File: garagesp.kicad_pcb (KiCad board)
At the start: 2 copper layers, 45 x 45 mm, 21 parts, among them J1 USB_C_Receptacle_USB2.0_14P, J2 AHT21, J3 DOOR CTL, J4 DOOR SW, K1 SANYOU_SRD_Form_A, Q1 BC547, SW1 RESET, SW2 BOOT, U1 ESP32-C3-WROOM-02, U2 AP2112K-3.3

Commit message: add capacitors and resistors
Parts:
- removed C1, C2: 10uF, Capacitor_SMD:C_0805_2012Metric_Pad1.18x1.45mm_HandSolder
- removed C3: 100 nF, Capacitor_SMD:C_0805_2012Metric_Pad1.18x1.45mm_HandSolder
- removed D1: B120-E3, Diode_SMD:D_SMA
- removed J1: USB_C_Receptacle_USB2.0_14P, Connector_USB:USB_C_Receptacle_HCTL_HC-TYPE-C-16P-01A
- removed J2: AHT21, Connector_PinHeader_2.54mm:PinHeader_1x04_P2.54mm_Vertical
- removed J3: DOOR CTL, Connector_Molex:Molex_Micro-Fit_3.0_43650-0200_1x02_P3.00mm_Horizontal
- removed J4: DOOR SW, Connector_Molex:Molex_Micro-Fit_3.0_43650-0200_1x02_P3.00mm_Horizontal
- removed K1: SANYOU_SRD_Form_A, Relay_THT:Relay_SPST_SANYOU_SRD_Series_Form_A
- removed Q1: BC547, Package_TO_SOT_THT:TO-92_Inline
- removed R1, R2, R7: 5.1k, Resistor_SMD:R_0805_2012Metric_Pad1.20x1.40mm_HandSolder
- removed R3, R4, R5, R6: 10k, Resistor_SMD:R_0805_2012Metric_Pad1.20x1.40mm_HandSolder
- removed SW1: RESET, Button_Switch_SMD:SW_SPST_TS-1088-xR020
- removed SW2: BOOT, Button_Switch_SMD:SW_SPST_TS-1088-xR020
- removed U1: ESP32-C3-WROOM-02, RF_Module:ESP32-C3-WROOM-02
- removed U2: AP2112K-3.3, Package_TO_SOT_SMD:SOT-23-5
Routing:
- net /3V3: track 59.7 -> 0.00 mm
- net GND: track 51.2 -> 0.00 mm, vias 1 -> 0
- net /SW: track 33.7 -> 0.00 mm
- net /5V: track 29.6 -> 0.00 mm, vias 3 -> 0
- net Net-(Q1-B): track 25.5 -> 0.00 mm
- net /CTL1: track 23.0 -> 0.00 mm
- net Net-(U1-EN): track 21.2 -> 0.00 mm
- net /CTL2: track 15.8 -> 0.00 mm
- net Net-(U1-IO2): track 13.5 -> 0.00 mm
- net Net-(U1-IO8): track 10.2 -> 0.00 mm
- net /SCL: track 9.87 -> 0.00 mm
- net /RELAY: track 9.21 -> 0.00 mm
- net Net-(D1-K): track 8.99 -> 0.00 mm
- net Net-(U1-IO9): track 8.86 -> 0.00 mm
- net /D+: track 7.56 -> 0.00 mm
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- removed copper zone on B.Cu, net GND
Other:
- board outline removed

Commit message: new pcb design
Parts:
- added C1: 10uF, Capacitor_SMD:C_0603_1608Metric_Pad1.08x0.95mm_HandSolder, F.Cu at (105.2, 71.5)
- added C10: 100nF, Capacitor_SMD:C_0603_1608Metric_Pad1.08x0.95mm_HandSolder, F.Cu at (98.6, 67.4)
- added C11: 4.7uF, Capacitor_SMD:CP_Elec_4x5.4, F.Cu at (103.0, 67.5)
- added C2: 10uF, Capacitor_SMD:C_0603_1608Metric_Pad1.08x0.95mm_HandSolder, F.Cu at (92.5, 69.0)
- added C3: 100nF, Capacitor_SMD:C_0603_1608Metric_Pad1.08x0.95mm_HandSolder, F.Cu at (90.8, 69.0)
- added C4: 10uF, Capacitor_SMD:C_0603_1608Metric_Pad1.08x0.95mm_HandSolder, F.Cu at (68.5, 51.8)
- added C5: 100nF, Capacitor_SMD:C_0603_1608Metric_Pad1.08x0.95mm_HandSolder, F.Cu at (66.5, 51.8)
- added C6: 10uF, Capacitor_SMD:C_0603_1608Metric_Pad1.08x0.95mm_HandSolder, F.Cu at (76.5, 69.5)
- added C7: 100nF, Capacitor_SMD:C_0603_1608Metric_Pad1.08x0.95mm_HandSolder, F.Cu at (78.2, 69.5)
- added C9: 10nF, Capacitor_SMD:C_0603_1608Metric_Pad1.08x0.95mm_HandSolder, F.Cu at (100.6, 61.2)
- added D1: B120-E3, Diode_SMD:D_SMA, F.Cu at (90.5, 72.5)
- added D2: RED LED, LED_SMD:LED_0603_1608Metric_Pad1.05x0.95mm_HandSolder, F.Cu at (108.8, 80.5)
- added D3: GREEN LED, LED_SMD:LED_0603_1608Metric_Pad1.05x0.95mm_HandSolder, F.Cu at (107.0, 80.5)
- added D4: GREEN LED, LED_SMD:LED_0603_1608Metric_Pad1.05x0.95mm_HandSolder, F.Cu at (69.4, 80.0)
- added D5: GREEN LED, LED_SMD:LED_0603_1608Metric_Pad1.05x0.95mm_HandSolder, F.Cu at (55.9, 76.2)
- added FB1: 70mΩ 33Ω@100MHz, Inductor_SMD:L_0805_2012Metric_Pad1.05x1.20mm_HandSolder, F.Cu at (98.6, 63.5)
- added J1: USB_C_Receptacle_USB2.0_14P, Connector_USB:USB_C_Receptacle_HCTL_HC-TYPE-C-16P-01A, F.Cu at (106.5, 58.0)
- added J2: AHT21, Connector_PinSocket_2.54mm:PinSocket_1x04_P2.54mm_Vertical, F.Cu at (62.5, 52.2)
- added J3: DOOR CTL, Connector_Molex:Molex_Micro-Fit_3.0_43650-0200_1x02_P3.00mm_Horizontal, F.Cu at (101.8, 85.4)
- added J4: DOOR SW, Connector_Molex:Molex_Micro-Fit_3.0_43650-0200_1x02_P3.00mm_Horizontal, F.Cu at (58.0, 85.4)
- added K1: SANYOU_SRD_Form_A, Relay_THT:Relay_SPST_SANYOU_SRD_Series_Form_A, F.Cu at (86.5, 76.0)
- added Q1: SS8050, Package_TO_SOT_SMD:SOT-23, F.Cu at (76.1, 81.5)
- added Q2: SS8050, Package_TO_SOT_SMD:SOT-23, F.Cu at (56.8, 79.2)
- added R1: 5.1k, Resistor_SMD:R_0603_1608Metric_Pad0.98x0.95mm_HandSolder, F.Cu at (103.4, 51.8)
- added R10: 1k, Resistor_SMD:R_0603_1608Metric_Pad0.98x0.95mm_HandSolder, F.Cu at (76.1, 78.7)
- added R11: 220, Resistor_SMD:R_0603_1608Metric_Pad0.98x0.95mm_HandSolder, F.Cu at (52.5, 79.0)
- added R12: 220, Resistor_SMD:R_0603_1608Metric_Pad0.98x0.95mm_HandSolder, F.Cu at (107.0, 77.0)
- added R13: 10k, Resistor_SMD:R_0603_1608Metric_Pad0.98x0.95mm_HandSolder, F.Cu at (52.5, 80.5)
- added R14: 220, Resistor_SMD:R_0603_1608Metric_Pad0.98x0.95mm_HandSolder, F.Cu at (108.8, 77.0)
- added R2: 5.1k, Resistor_SMD:R_0603_1608Metric_Pad0.98x0.95mm_HandSolder, F.Cu at (103.4, 64.2)
- added R3: 10k, Resistor_SMD:R_0603_1608Metric_Pad0.98x0.95mm_HandSolder, F.Cu at (76.5, 66.0)
- added R4: 10k, Resistor_SMD:R_0603_1608Metric_Pad0.98x0.95mm_HandSolder, F.Cu at (83.8, 66.0)
- added R5: 10k, Resistor_SMD:R_0603_1608Metric_Pad0.98x0.95mm_HandSolder, F.Cu at (78.2, 66.0)
- added R6: 10k, Resistor_SMD:R_0603_1608Metric_Pad0.98x0.95mm_HandSolder, F.Cu at (73.8, 65.1)
- added R7: 100, Resistor_SMD:R_0603_1608Metric_Pad0.98x0.95mm_HandSolder, F.Cu at (67.5, 61.8)
- added R8: 2.2k, Resistor_SMD:R_0603_1608Metric_Pad0.98x0.95mm_HandSolder, F.Cu at (58.8, 59.9)
- added R9: 2.2k, Resistor_SMD:R_0603_1608Metric_Pad0.98x0.95mm_HandSolder, F.Cu at (58.8, 57.3)
- added SW1: ~, Button_Switch_SMD:SW_SPST_TS-1088-xR020, F.Cu at (81.0, 69.0)
- added SW2: ~, Button_Switch_SMD:SW_SPST_TS-1088-xR020, F.Cu at (73.8, 69.0)
- added U1: ESP32-C3-WROOM-02, RF_Module:ESP32-C3-WROOM-02, F.Cu at (79.4, 56.8)
- added U2: AMS1117-3.3, Package_TO_SOT_SMD:SOT-223-3_TabPin2, F.Cu at (99.0, 73.8)
- added U3: USBLC6-2SC6, Package_TO_SOT_SMD:SOT-23-6, F.Cu at (97.6, 58.0)
- added U4: PC817, Package_DIP:DIP-4_W7.62mm, F.Cu at (69.4, 73.7)
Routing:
- net +3V3: track 0.00 -> 114.7 mm
- net /SW: track 0.00 -> 28.7 mm
- net /EN: track 0.00 -> 24.8 mm
- net /CTL2: track 0.00 -> 20.3 mm
- net /CTL1: track 0.00 -> 19.2 mm
- net +5V: track 0.00 -> 17.9 mm
- net Net-(U3-VBUS): track 0.00 -> 16.8 mm
- net Net-(D1-A): track 0.00 -> 15.1 mm
- net Net-(U1-IO2): track 0.00 -> 13.5 mm
- net /SDA: track 0.00 -> 12.9 mm
- net GND: track 0.00 -> 12.9 mm, vias 0 -> 41
- net /BOOT: track 0.00 -> 12.5 mm
- net /SCL: track 0.00 -> 12.4 mm
- net Net-(R7-Pad1): track 0.00 -> 11.9 mm
- net Net-(U1-IO18): track 0.00 -> 8.63 mm
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- added copper zone on B.Cu, net GND
- added copper zone on F.Cu, net GND
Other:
- board outline added: 60 x 45 mm

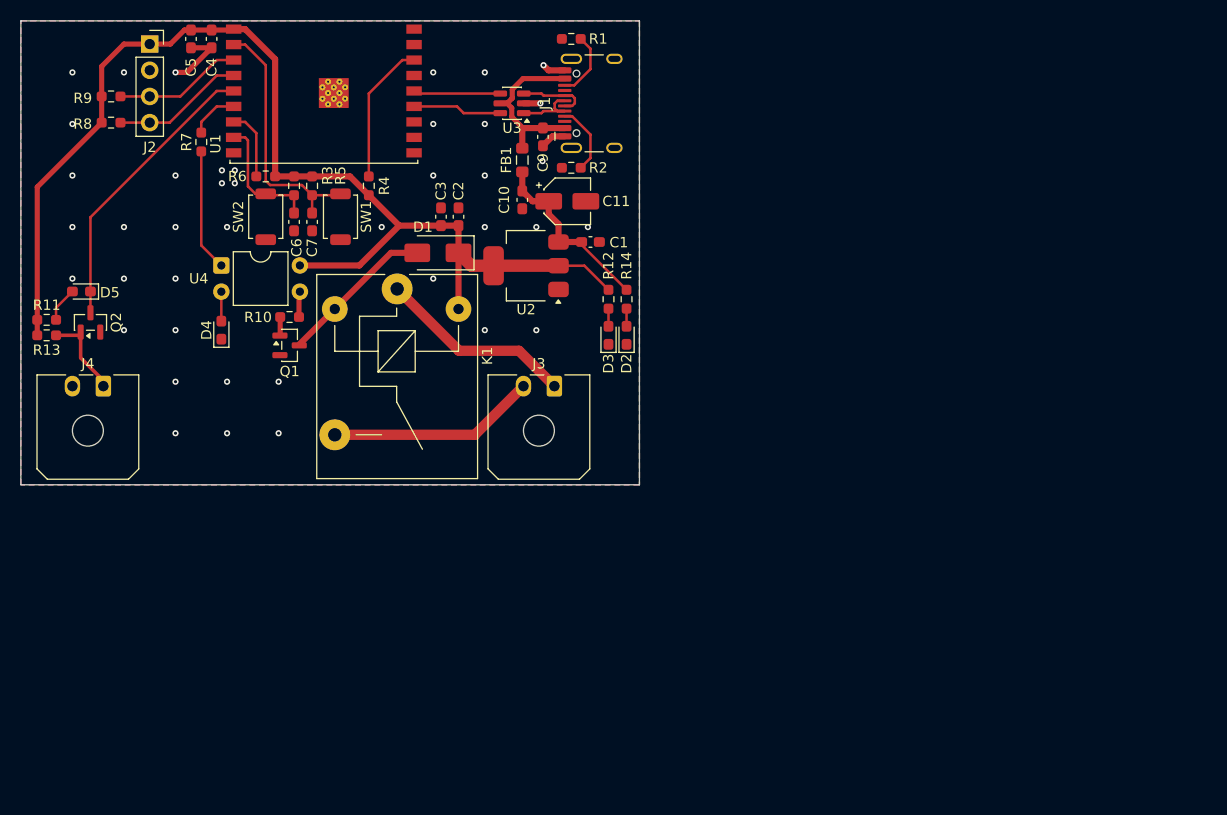
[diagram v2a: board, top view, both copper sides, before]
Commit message: I like this but want to invert my input LEDs
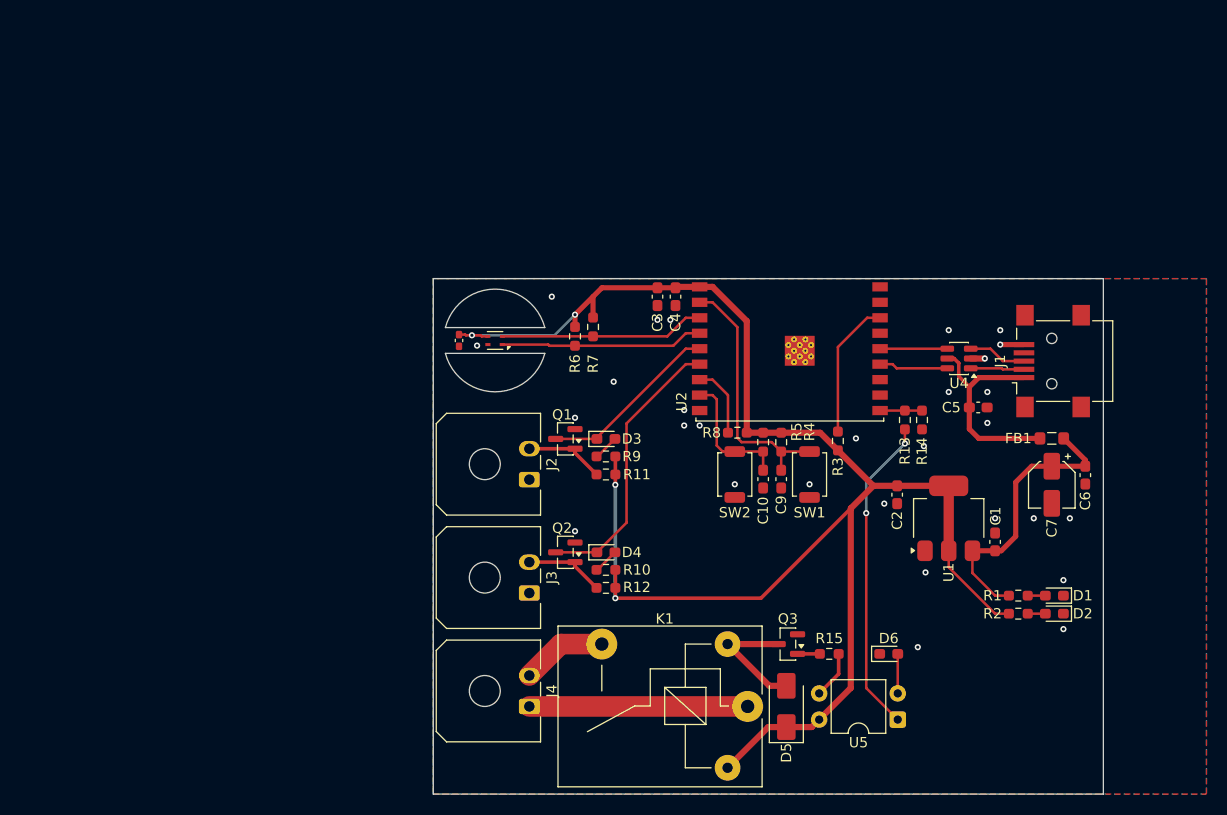
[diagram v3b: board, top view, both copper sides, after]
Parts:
- removed the C3 at (90.8, 69.0)
- removed the R1 at (103.4, 51.8)
- removed the R10 at (76.1, 78.7)
- removed the R2 at (103.4, 64.2)
- added C8: 100nF, Capacitor_SMD:C_0402_1005Metric_Pad0.74x0.62mm_HandSolder, F.Cu at (92.5, 81.0)
- added D3: GREEN LED, LED_SMD:LED_0603_1608Metric_Pad1.05x0.95mm_HandSolder, F.Cu at (106.8, 90.5)
- added Q1: SS8050, Package_TO_SOT_SMD:SOT-23, F.Cu at (102.8, 90.5)
- added R11: 10k, Resistor_SMD:R_0603_1608Metric_Pad0.98x0.95mm_HandSolder, F.Cu at (106.8, 94.0)
- added R14: 10k, Resistor_SMD:R_0603_1608Metric_Pad0.98x0.95mm_HandSolder, F.Cu at (137.4, 88.7)
- added R15: 1k, Resistor_SMD:R_0603_1608Metric_Pad0.98x0.95mm_HandSolder, F.Cu at (128.4, 111.4)
- added R9: 220, Resistor_SMD:R_0603_1608Metric_Pad0.98x0.95mm_HandSolder, F.Cu at (106.8, 92.2)
- added U3: SHT4x, Sensor_Humidity:Sensirion_DFN-4_1.5x1.5mm_P0.8mm_SHT4x_NoCentralPad, F.Cu at (96.0, 81.0)
- C2: value 10uF -> 22uF
- J1: value USB_C_Receptacle_USB2.0_14P -> USB_B_Mini; footprint Connector_USB:USB_C_Receptacle_HCTL_HC-TYPE-C-16P-01A -> Connector_USB:USB_Mini-B_Lumberg_2486_01_Horizontal
- J2: value AHT21 -> ~; footprint Connector_PinSocket_2.54mm:PinSocket_1x04_P2.54mm_Vertical -> Connector_Molex:Molex_Micro-Fit_3.0_43650-0200_1x02_P3.00mm_Horizontal
- J3: renamed from J4; value DOOR SW -> ~
- J4: renamed from J3; value DOOR CTL -> ~
- moved U5 79.0 mm to (135.1, 117.8), turned to 180 degrees
- moved R13 73.4 mm to (135.8, 88.7)
- moved D6 71.9 mm to (134.2, 111.4), turned to 0 degrees
- moved C6 60.8 mm to (153.2, 94.1)
- moved R12 59.5 mm to (106.8, 105.0), turned to 0 degrees
- moved R10 59.4 mm to (106.8, 103.2), turned to 180 degrees
- moved FB1 58.0 mm to (150.0, 90.5), turned to 180 degrees
- moved D4 56.8 mm to (106.8, 101.5), turned to 0 degrees
- moved Q3 56.4 mm to (124.4, 110.5), turned to 180 degrees
- moved J2 56.0 mm to (99.3, 94.5), turned to 90 degrees
- moved D5 55.5 mm to (124.2, 116.5), turned to 90 degrees
- moved C7 54.5 mm to (150.0, 95.0), turned to -90 degrees
- moved C9 53.4 mm to (123.8, 94.5)
- moved R4 53.4 mm to (123.8, 90.9)
- moved K1 52.9 mm to (120.5, 116.5), turned to 180 degrees
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- renumbered C7 to C10, C5 to C3, C9 to C5, C10 to C6, C11 to C7, C6 to C9, D2 to D1, D3 to D2, D5 to D4, D1 to D5, D4 to D6, Q1 to Q3, R14 to R1, R11 to R10, R13 to R12, R7 to R13, R12 to R2, R4 to R3, R3 to R4, R8 to R6, R9 to R7, R6 to R8, U2 to U1, U1 to U2, U3 to U4, U4 to U5
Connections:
- C10 pad 2: /EN -> BOOT
- C5 pad 1: Net-(U3-VBUS) -> Net-(J1-VBUS)
- C9 pad 1: /BOOT -> EN
- D4 pad 1: /SW -> IN2
- FB1 pad 2: Net-(U3-VBUS) -> Net-(J1-VBUS)
- J2 pad 1: +3V3 -> GND
- J2 pad 2: GND -> Net-(J2-Pin_2)
- J3 pad 1: Net-(J4-Pin_1) -> GND
- J3 pad 2: GND -> Net-(J3-Pin_2)
- Q2 pad 1: Net-(J4-Pin_1) -> Net-(J3-Pin_2)
- Q2 pad 3: /SW -> IN2
- R12 pad 1: Net-(J4-Pin_1) -> Net-(J3-Pin_2)
- R13 pad 2: /RELAY -> RELAY
- R4 pad 1: /BOOT -> EN
- R5 pad 1: /EN -> BOOT
- R6 pad 1: /SDA -> SDA
- R7 pad 1: /SCL -> SCL
- SW1 pad 2: /EN -> EN
- SW2 pad 2: /BOOT -> BOOT
- U2 pad 10: unconnected-(U1-IO10-Pad10) -> RELAY
- U2 pad 2: /EN -> EN
- U2 pad 3: /SCL -> SCL
- U2 pad 4: /SDA -> SDA
- U2 pad 5: /SW -> IN1
- U2 pad 6: /RELAY -> IN2
- U2 pad 8: /BOOT -> BOOT
- U4 pad 1: Net-(J1-D--PadA7) -> Net-(J1-D-)
- U4 pad 3: Net-(J1-D+-PadA6) -> Net-(J1-D+)
- U4 pad 5: Net-(U3-VBUS) -> Net-(J1-VBUS)
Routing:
- net +3V3: track 114.7 -> 162.8 mm, vias 0 -> 4
- net /SW: track 28.7 -> 0.00 mm
- net IN2: track 0.00 -> 27.2 mm
- net EN: track 0.00 -> 25.9 mm
- net /EN: track 24.8 -> 0.00 mm
- net Net-(J1-VBUS): track 0.00 -> 21.0 mm
- net SCL: track 0.00 -> 19.9 mm
- net SDA: track 0.00 -> 19.7 mm
- net Net-(R13-Pad1): track 11.9 -> 31.0 mm, vias 0 -> 2
- net IN1: track 0.00 -> 17.7 mm
- net Net-(U3-VBUS): track 16.8 -> 0.00 mm
- net BOOT: track 0.00 -> 12.9 mm
- net /SDA: track 12.9 -> 0.00 mm
- net /BOOT: track 12.5 -> 0.00 mm
- net /SCL: track 12.4 -> 0.00 mm
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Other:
- board size 60 x 45 mm -> 65 x 50 mm
